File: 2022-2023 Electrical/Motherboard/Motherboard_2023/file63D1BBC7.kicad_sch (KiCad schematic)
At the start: 9 parts, among them J11 Conn_01x06_Male, J12 VCF4-1000, J13 VCF4-1000, J14 Conn_01x03_Male, J15 VCF4-1000, J16 VCF4-1000, J17 Conn_01x02_Male, Q2 Q_NMOS_GDS

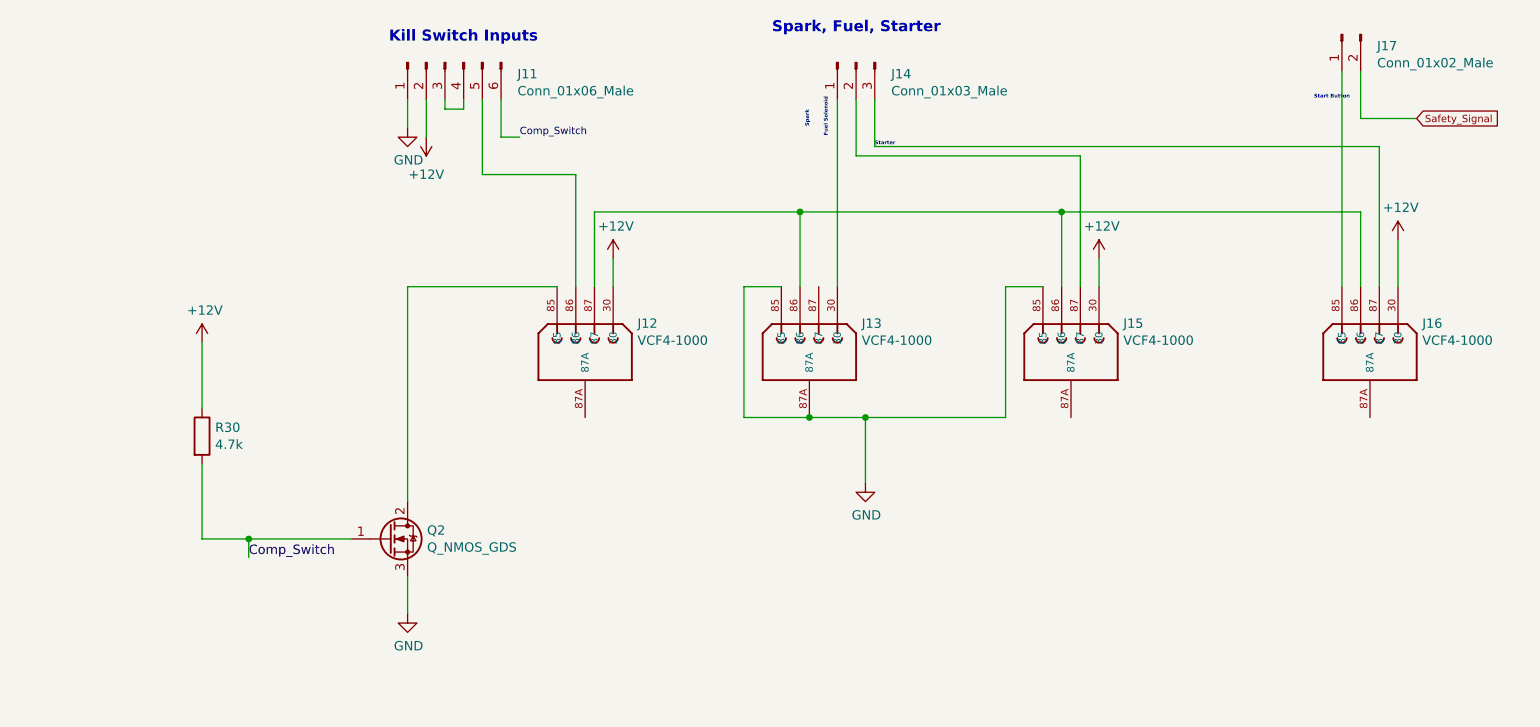
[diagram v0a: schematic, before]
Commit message: Added BOM
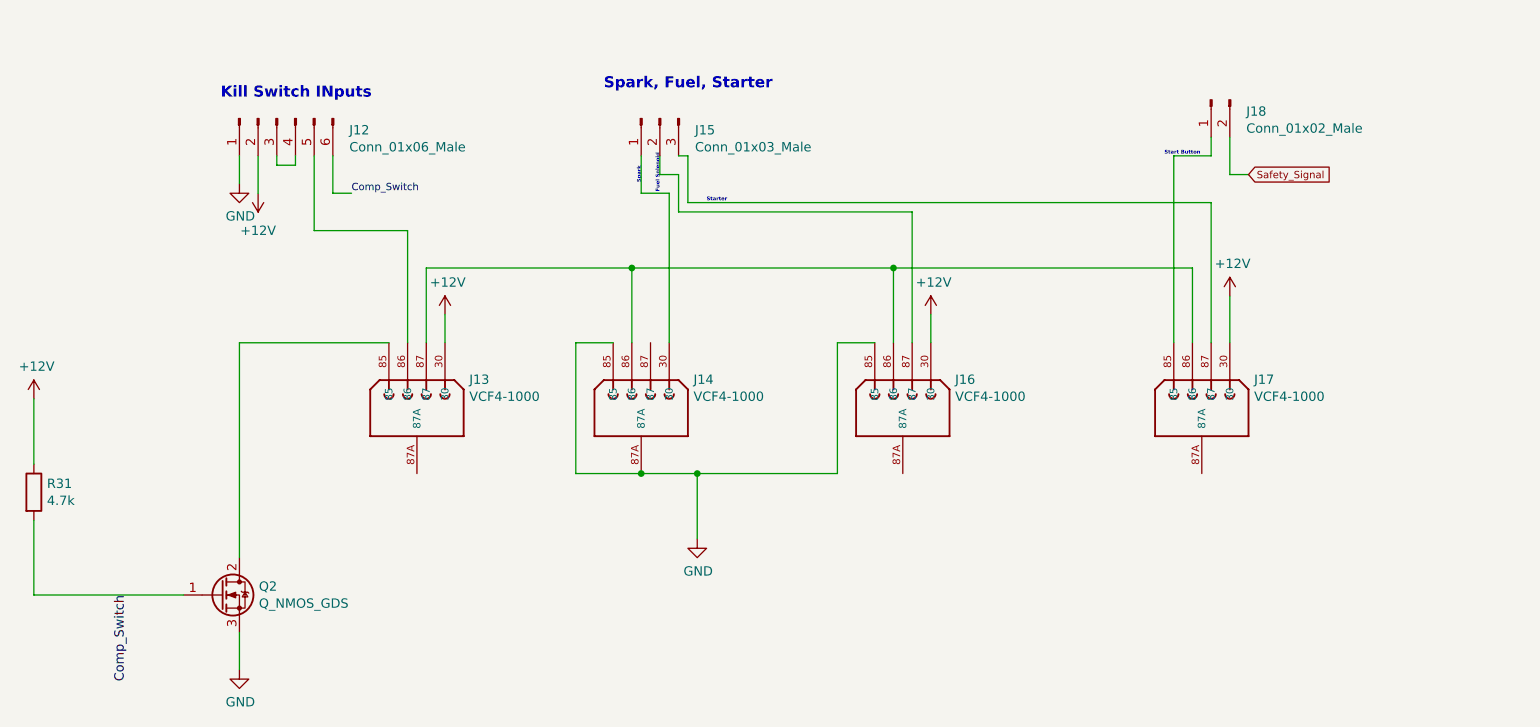
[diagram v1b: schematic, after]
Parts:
- removed J11: Conn_01x06_Male, TerminalBlock_Phoenix:TerminalBlock_Phoenix_MKDS-3-6-5.08_1x06_P5.08mm_Horizontal, symbol Motherboard_2023-rescue:Conn_01x06_Male-Connector
- removed J12, J15: VCF4-1000, VCF4-1000 (Relay Socket):TE_VCF4-1000, symbol Motherboard_2023-rescue:VCF4-1000-VCF4-1000-Motherboard_2023-rescue
- removed J14: Conn_01x03_Male, TerminalBlock_Phoenix:TerminalBlock_Phoenix_MKDS-3-3-5.08_1x03_P5.08mm_Horizontal, symbol Motherboard_2023-rescue:Conn_01x03_Male-Connector
- removed J17: Conn_01x02_Male, TerminalBlock_Phoenix:TerminalBlock_Phoenix_MKDS-1,5-2-5.08_1x02_P5.08mm_Horizontal, symbol Motherboard_2023-rescue:Conn_01x02_Male-Connector
- removed R30: 4.7k, Resistor_THT:R_Axial_DIN0207_L6.3mm_D2.5mm_P10.16mm_Horizontal, symbol Device:R
- added J12: Conn_01x06_Male, TerminalBlock_Phoenix:TerminalBlock_Phoenix_MKDS-3-6-5.08_1x06_P5.08mm_Horizontal, symbol Motherboard_2023-rescue:Conn_01x06_Male-Connector
- added J14, J17: VCF4-1000, VCF4-1000 (Relay Socket):TE_VCF4-1000, symbol Motherboard_2023-rescue:VCF4-1000-VCF4-1000-Motherboard_2023-rescue
- added J15: Conn_01x03_Male, TerminalBlock_Phoenix:TerminalBlock_Phoenix_MKDS-3-3-5.08_1x03_P5.08mm_Horizontal, symbol Motherboard_2023-rescue:Conn_01x03_Male-Connector
- added J18: Conn_01x02_Male, TerminalBlock_Phoenix:TerminalBlock_Phoenix_MKDS-1,5-2-5.08_1x02_P5.08mm_Horizontal, symbol Motherboard_2023-rescue:Conn_01x02_Male-Connector
- added R31: 4.7k, Resistor_THT:R_Axial_DIN0207_L6.3mm_D2.5mm_P10.16mm_Horizontal, symbol Device:R
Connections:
- net +12V: now also J13.30, J12.2 (Pin_2), J17.30, R31.1
- net Comp_Switch: now also J12.6 (Pin_6), R31.2
- net GND: now also J16.85, J12.1 (Pin_1), J14.85, J14.87A; no longer J13.85, J13.87A
- net Safety_Signal: now also J18.2 (Pin_2)
- net at Q2.2 (D): now also J13.85
- net at J13.86: now also J12.5 (Pin_5); no longer J16.86
- net at J16.87: now also J15.2 (Pin_2)
- net at J13.87: now also J16.86, J14.86, J17.86
- new net: J14.30, J15.1 (Pin_1)
- new net: J17.85, J18.1 (Pin_1)
- new net: J15.3 (Pin_3), J17.87
- new net: J12.3 (Pin_3), J12.4 (Pin_4)
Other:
- note added: "Kill Switch INputs"
- note removed: "Kill Switch Inputs"
